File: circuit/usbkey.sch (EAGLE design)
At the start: 30 parts, among them IC1 ATmega168P, P1 SPEAKER, P2 LED, P3 OUTPUT, Q1 18MHz, X1 1503_09, X2 USB

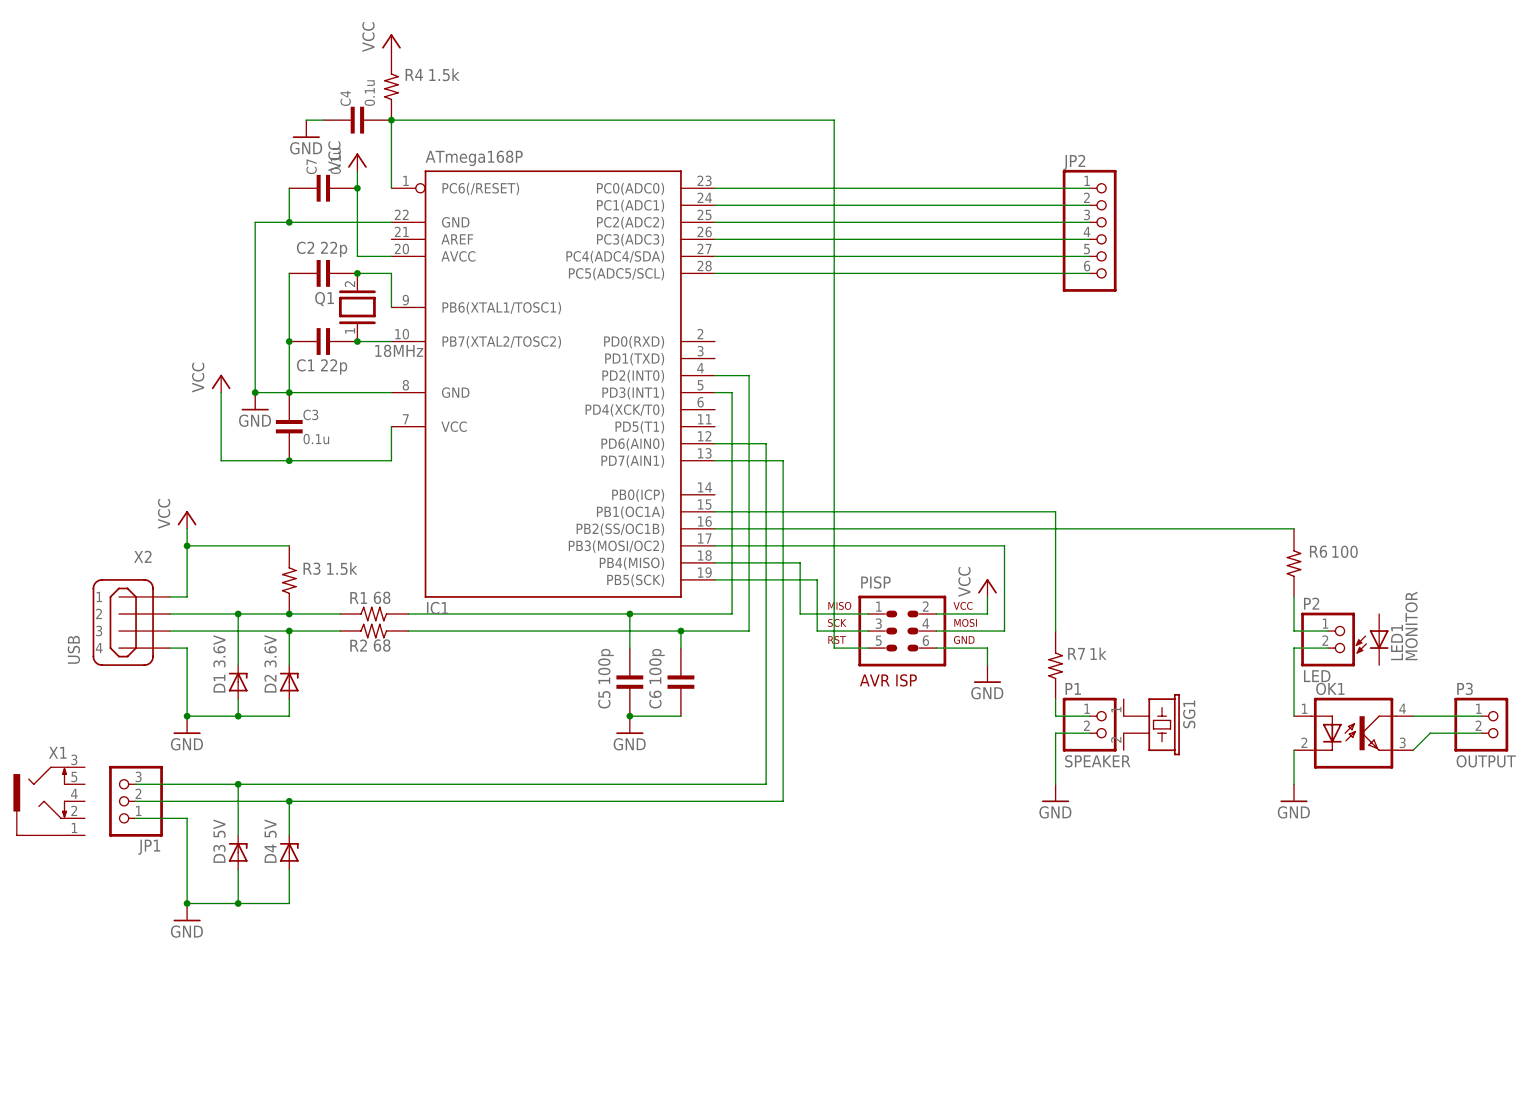
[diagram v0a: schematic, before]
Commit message: update
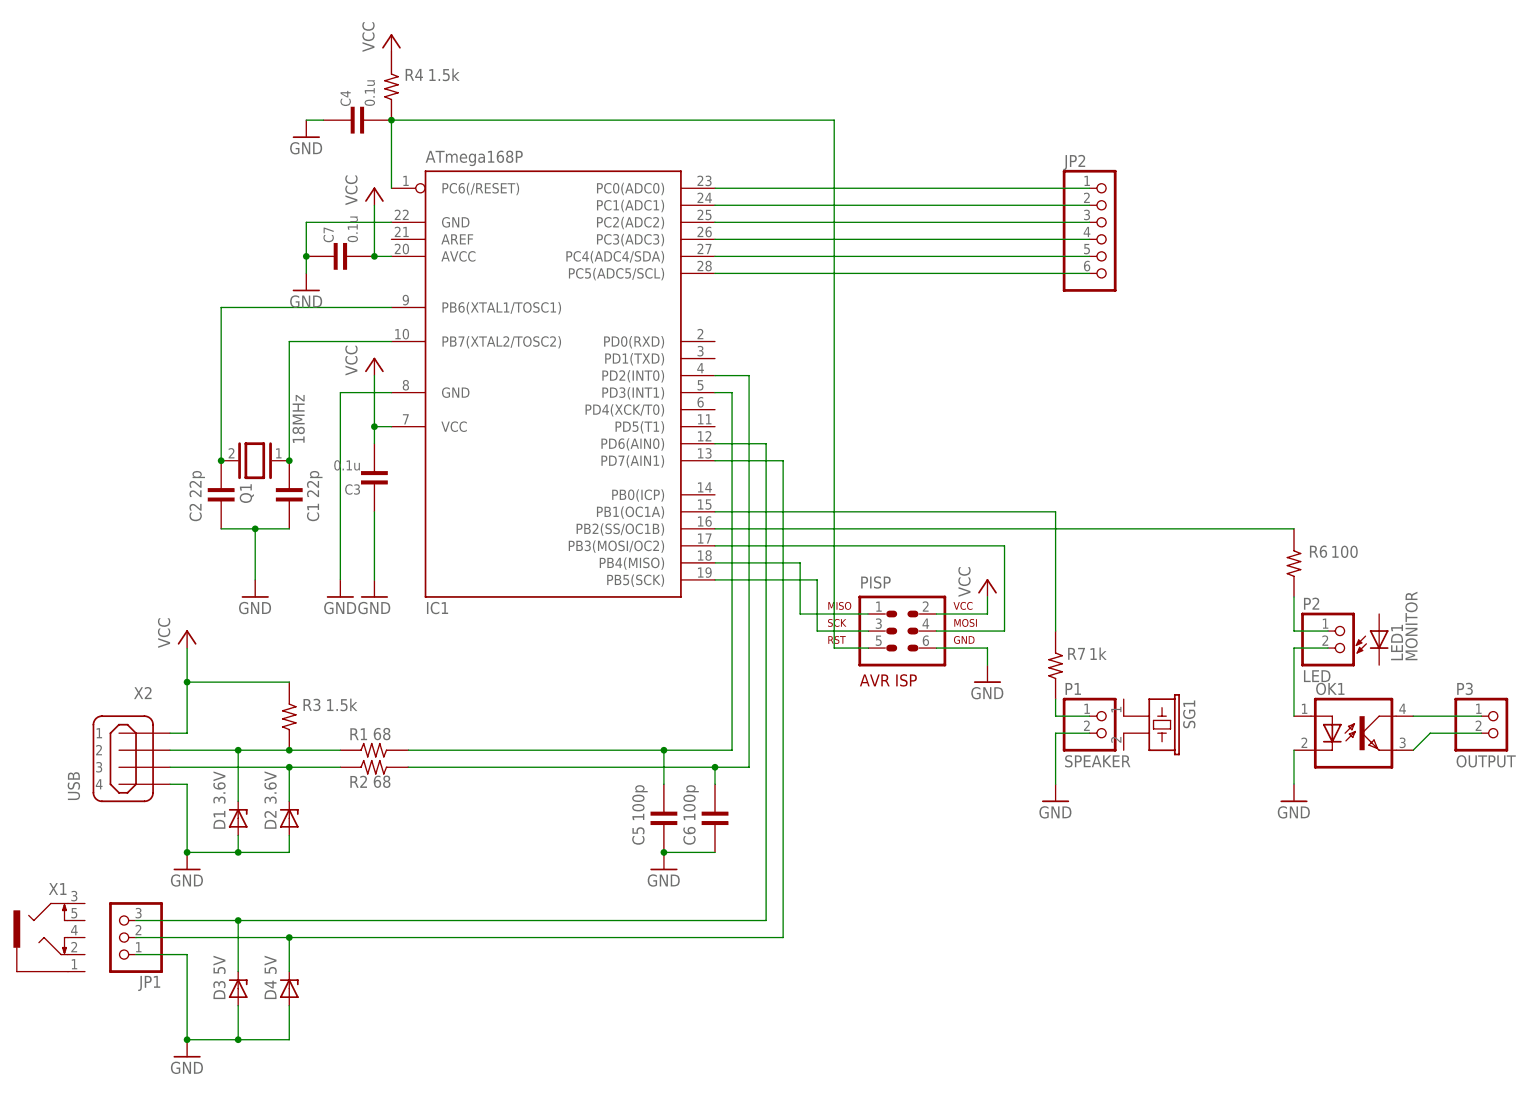
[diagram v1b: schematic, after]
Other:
- moved on the sheet: C1, C2, C3, C5, C6, C7, D1, D2, D3, D4, JP1, Q1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
